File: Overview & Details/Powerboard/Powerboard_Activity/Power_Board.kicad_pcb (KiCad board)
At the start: 4 copper layers, 198 x 120.6 mm, 51 parts, among them J1 Jack-DC, J2 Screw_Terminal_01x04, J3 Screw_Terminal_01x04, J4 Screw_Terminal_01x02, J5 Screw_Terminal_01x02, U1 LM2576S-ADJ, U2 LM2576S-ADJ, U3 LM2576S-ADJ, U4 LM2576S-ADJ, U5 MAX735CSA

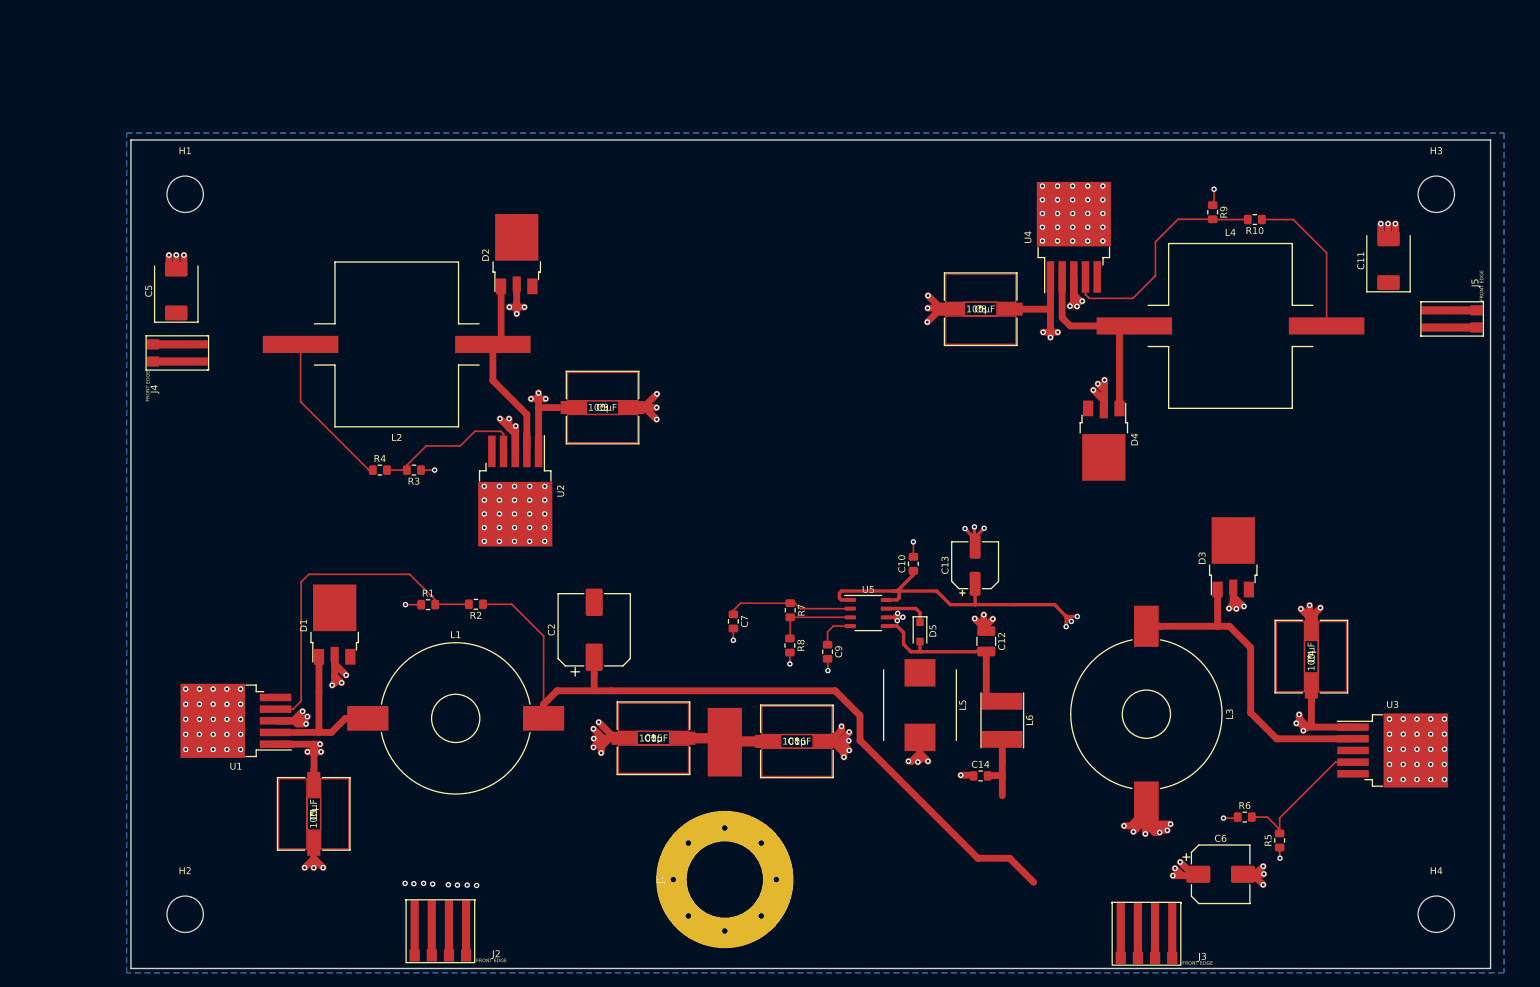
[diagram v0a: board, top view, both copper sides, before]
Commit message: Finish powerboard design
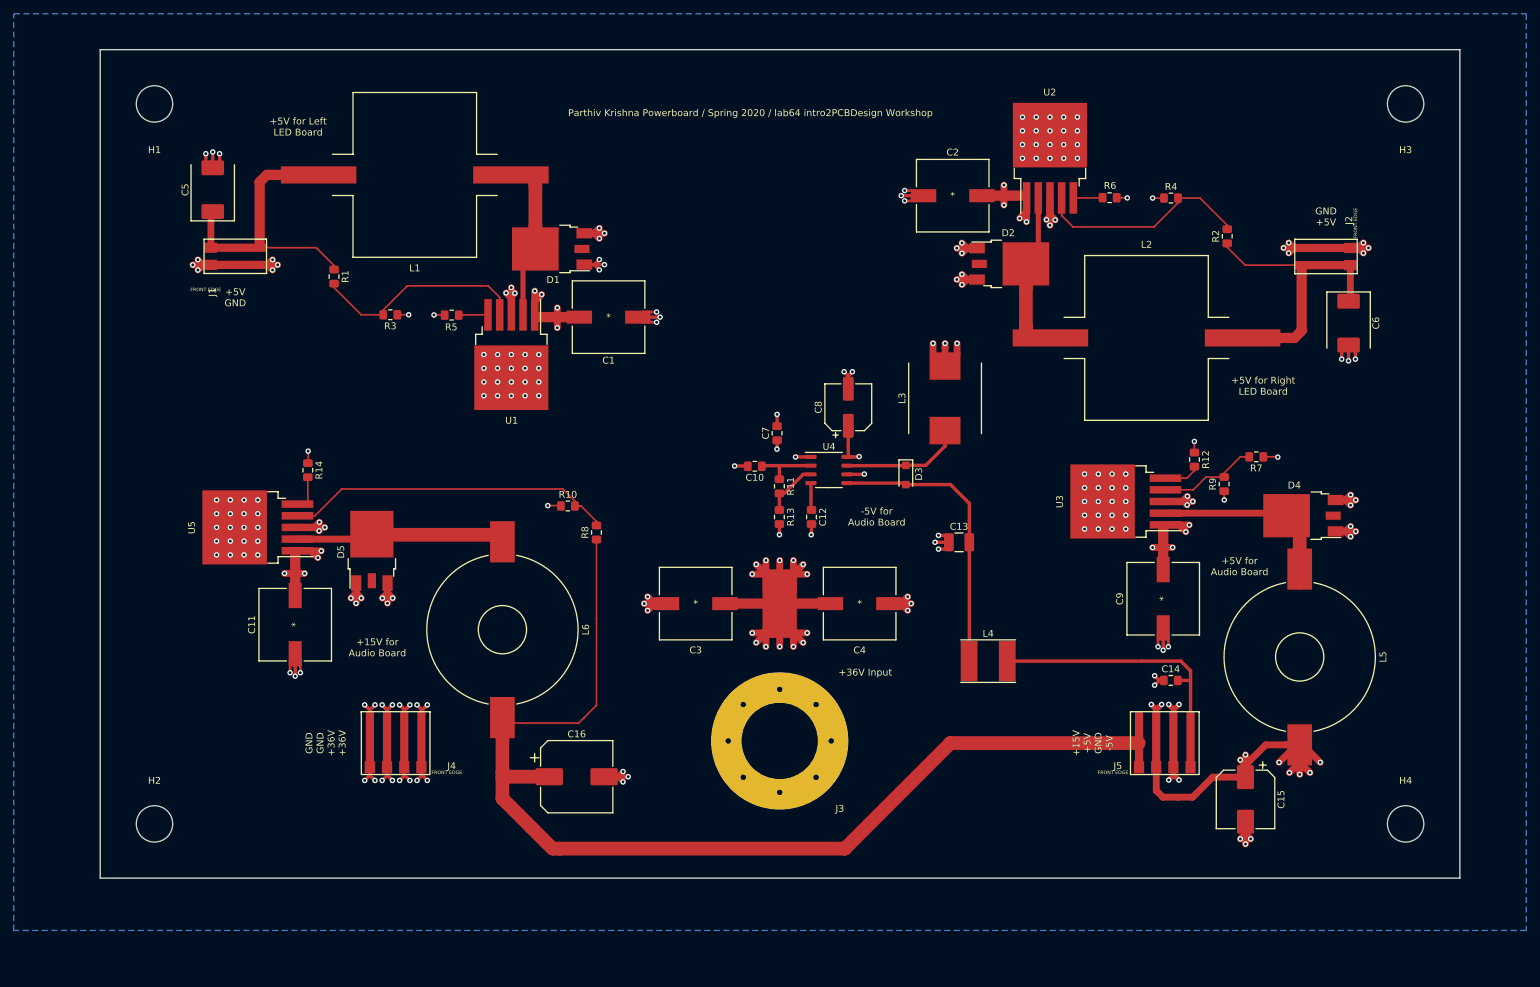
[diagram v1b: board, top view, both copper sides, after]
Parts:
- added R11: 130kΩ, Resistor_SMD:R_0805_2012Metric_Pad1.15x1.40mm_HandSolder, F.Cu at (149.0, 97.4)
- added R12: 20kΩ, Resistor_SMD:R_0805_2012Metric_Pad1.15x1.40mm_HandSolder, F.Cu at (209.5, 93.5)
- added R13: 300kΩ, Resistor_SMD:R_0805_2012Metric_Pad1.15x1.40mm_HandSolder, F.Cu at (149.0, 101.9)
- added R14: 20kΩ, Resistor_SMD:R_0805_2012Metric_Pad1.15x1.40mm_HandSolder, F.Cu at (80.4, 95.1)
- C10: value 1μF@10V -> 10μF@16V
- C11: value 1000µF -> 100µF; footprint Capacitor_Tantalum_SMD:CP_EIA-7361-438_AVX-U_Pad2.18x3.30mm_HandSolder -> Powerboard:PCR1J101MCL1GS
- C12: value 100μF@10V -> 82pF; footprint Capacitor_SMD:C_1210_3225Metric_Pad1.42x2.65mm_HandSolder -> Capacitor_SMD:C_0805_2012Metric_Pad1.15x1.40mm_HandSolder
- C13: value 47μF@10V -> 100μF@10V; footprint Capacitor_SMD:CP_Elec_6.3x5.7 -> Capacitor_SMD:C_1210_3225Metric_Pad1.42x2.65mm_HandSolder
- C15: value 100μF -> 330µF; footprint Powerboard:PCR1J101MCL1GS -> Capacitor_SMD:CP_Elec_8x10
- C16: value 100μF -> 68µF; footprint Powerboard:PCR1J101MCL1GS -> Capacitor_SMD:CP_Elec_10x10
- C2: value 68µF -> 100µF; footprint Capacitor_SMD:CP_Elec_10x10 -> Powerboard:PCR1J101MCL1GS
- C3, C4: value 100µF -> 100μF
- C6: value 330µF -> 1000µF; footprint Capacitor_SMD:CP_Elec_8x10 -> Capacitor_Tantalum_SMD:CP_EIA-7361-438_AVX-U_Pad2.18x3.30mm_HandSolder
- C7: value 10μF@16V -> 1μF@10V
- C8: value 100µF -> 47μF@10V; footprint Powerboard:PCR1J101MCL1GS -> Capacitor_SMD:CP_Elec_6.3x5.7
- C9: value 82pF -> 100µF; footprint Capacitor_SMD:C_0805_2012Metric_Pad1.15x1.40mm_HandSolder -> Powerboard:PCR1J101MCL1GS
- D3: value VS-MURD620CT-M3 -> PMEG2010AEH; footprint Powerboard:TO-252AA_TabPin4 -> Diode_SMD:D_SOD-123F
- D5: value PMEG2010AEH -> VS-MURD620CT-M3; footprint Diode_SMD:D_SOD-123F -> Powerboard:TO-252AA_TabPin4
- J1: value Jack-DC -> Screw_Terminal_01x02; footprint Powerboard:BarrelJack_Power_2.1x5.5mm_11mmThruHole_PanelMount -> Powerboard:AVX-Wire-To-Board-1x2
- J2: value Screw_Terminal_01x04 -> Screw_Terminal_01x02; footprint Powerboard:AVX-Wire-To-Board-1x4 -> Powerboard:AVX-Wire-To-Board-1x2
- J3: value Screw_Terminal_01x04 -> Jack-DC; footprint Powerboard:AVX-Wire-To-Board-1x4 -> Powerboard:BarrelJack_Power_2.1x5.5mm_11mmThruHole_PanelMount
- J4, J5: value Screw_Terminal_01x02 -> Screw_Terminal_01x04; footprint Powerboard:AVX-Wire-To-Board-1x2 -> Powerboard:AVX-Wire-To-Board-1x4
- L1: value 470µH -> 100µH; footprint Powerboard:L_Toroid_Horizontal_D21.8mm_P19.60mm_Bourns_2100 -> Powerboard:Eaton_CTX100-2-52-R
- L3: value 330µH -> 10μH; footprint Powerboard:L_Toroid_Horizontal_D21.8mm_P19.60mm_Bourns_2100 -> Powerboard:L_Taiyo-Yuden_NR-10050_9.8x10.0mm_HandSoldering
- L4: value 100µH -> 22μH; footprint Powerboard:Eaton_CTX100-2-52-R -> Powerboard:L_Taiyo-Yuden_NR-60xx_HandSoldering
- L5: value 10μH -> 330µH; footprint Powerboard:L_Taiyo-Yuden_NR-10050_9.8x10.0mm_HandSoldering -> Powerboard:L_Toroid_Horizontal_D21.8mm_P19.60mm_Bourns_2100
- L6: value 22μH -> 470µH; footprint Powerboard:L_Taiyo-Yuden_NR-60xx_HandSoldering -> Powerboard:L_Toroid_Horizontal_D21.8mm_P19.60mm_Bourns_2100
- R1: value 1.02kΩ -> 3.09kΩ
- R10: value 3.09kΩ -> 1.02kΩ
- R2: value 11.50kΩ -> 3.09kΩ
- R4: value 3.09kΩ -> 1.0kΩ
- R5: value 1.0kΩ -> 20kΩ
- R6: value 3.09kΩ -> 20kΩ
- R7: value 130kΩ -> 3.09kΩ
- R8: value 300kΩ -> 11.50kΩ
- U4: value LM2576S-ADJ -> MAX735CSA; footprint Package_TO_SOT_SMD:TO-263-5_TabPin3 -> Package_SO:SOP-8_3.9x4.9mm_P1.27mm
- U5: value MAX735CSA -> LM2576S-ADJ; footprint Package_SO:SOP-8_3.9x4.9mm_P1.27mm -> Package_TO_SOT_SMD:TO-263-5_TabPin3
- moved J2 169.3 mm to (232.2, 65.2), turned to 90 degrees
- moved C11 167.8 mm to (78.5, 117.6), turned to 270 degrees
- moved R5 142.8 mm to (101.3, 72.5), turned to 0 degrees
- moved R2 121.8 mm to (214.3, 61.0), turned to 90 degrees
- moved R4 121.8 mm to (206.1, 55.4)
- moved J1 118.6 mm to (66.3, 62.7), turned to 270 degrees
- moved L2 109.2 mm to (202.5, 75.8), turned to 0 degrees
- moved R10 108.4 mm to (118.2, 100.3), turned to 0 degrees
- moved R6 92.3 mm to (197.1, 55.4), turned to 180 degrees
- moved U2 91.7 mm to (188.4, 49.7), turned to 90 degrees
- moved U5 89.8 mm to (73.1, 103.4), turned to 180 degrees
- moved C15 86.7 mm to (216.9, 143.0), turned to 270 degrees
- moved C1 84.1 mm to (124.2, 72.8), turned to 0 degrees
- moved C6 82.4 mm to (231.9, 73.7), turned to 270 degrees
- moved C2 82.0 mm to (174.3, 55.1), turned to 180 degrees
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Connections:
- C10 pad 1: +5VA -> Net-(C10-Pad1)
- C11 pad 1: +5VR -> +36V
- C12 pad 1: GNDS -> Net-(C12-Pad1)
- C12 pad 2: Net-(C12-Pad2) -> GNDS
- C13 pad 1: +5VA -> GNDS
- C13 pad 2: GNDS -> Net-(C13-Pad2)
- C15 pad 1: +36V -> +5VA
- C16 pad 1: +36V -> +15V
- C2 pad 1: +15V -> +36V
- C6 pad 1: +5VA -> +5VR
- C7 pad 1: Net-(C7-Pad1) -> +5VA
- C8 pad 1: +36V -> +5VA
- C9 pad 1: Net-(C9-Pad1) -> +36V
- D3 pad 2: GNDS -> Net-(C13-Pad2)
- D5 pad 2: Net-(C12-Pad2) -> GNDS
- J1 pad 1: GNDS -> +5VL
- J1 pad 2: +36V -> GNDS
- J2 pad : (no net) -> +5VR
- J2 pad 1: GNDS -> +5VR
- J3 pad 1: +15V -> GNDS
- J3 pad 2: +5VA -> +36V
- J4 pad : (no net) -> GNDS
- J4 pad 1: +5VL -> GNDS
- J5 pad : (no net) -> -5VA
- J5 pad 1: +5VR -> +15V
- J5 pad 2: GNDS -> +5VA
- J5 pad 3: (no net) -> GNDS
- J5 pad 4: (no net) -> -5VA
- L1 pad 2: +15V -> +5VL
- L2 pad 2: +5VL -> +5VR
- L3 pad 2: +5VA -> GNDS
- L4 pad 1: Net-(D4-Pad1) -> Net-(C13-Pad2)
- L4 pad 2: +5VR -> -5VA
- L5 pad 1: Net-(D5-Pad1) -> Net-(D4-Pad1)
- L5 pad 2: GNDS -> +5VA
- L6 pad 1: Net-(C12-Pad2) -> Net-(D5-Pad1)
- L6 pad 2: -5VA -> +15V
- R1 pad 1: GNDS -> +5VL
- R10 pad 1: +5VR -> GNDS
- R2 pad 1: +15V -> +5VR
- R2 pad 2: Net-(R1-Pad2) -> Net-(R2-Pad2)
- R3 pad 2: Net-(R3-Pad2) -> Net-(R1-Pad2)
- R4 pad 1: +5VL -> GNDS
- R4 pad 2: Net-(R3-Pad2) -> Net-(R2-Pad2)
- R6 pad 1: +5VA -> GNDS
- R6 pad 2: Net-(R5-Pad2) -> Net-(R6-Pad2)
- R7 pad 1: Net-(C7-Pad1) -> +5VA
- R8 pad 1: Net-(R7-Pad2) -> +15V
- R8 pad 2: GNDS -> Net-(R10-Pad2)
- R9 pad 2: Net-(R10-Pad2) -> Net-(R7-Pad2)
- U1 pad 5: Net-(U1-Pad5) -> Net-(R5-Pad2)
- U2 pad 4: Net-(R3-Pad2) -> Net-(R2-Pad2)
- U2 pad 5: Net-(U2-Pad5) -> Net-(R6-Pad2)
- U3 pad 2: Net-(D3-Pad1) -> Net-(D4-Pad1)
- U3 pad 4: Net-(R5-Pad2) -> Net-(R7-Pad2)
- U4 pad 1: +36V -> +5VA
- U4 pad 2: Net-(D4-Pad1) -> Net-(C10-Pad1)
- U4 pad 3: GNDS -> Net-(R11-Pad2)
- U4 pad 4: Net-(R10-Pad2) -> Net-(C12-Pad1)
- U4 pad 5: Net-(U4-Pad5) -> Net-(C13-Pad2)
- U5 pad 1: +5VA -> +36V
- U5 pad 2: Net-(C7-Pad1) -> Net-(D5-Pad1)
- U5 pad 3: Net-(R7-Pad2) -> GNDS
- U5 pad 4: Net-(C9-Pad1) -> Net-(R10-Pad2)
- U5 pad 5: Net-(C12-Pad2) -> Net-(R14-Pad2)
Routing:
- net +36V: track 78.1 -> 193.2 mm, vias 16 -> 38
- net GNDS: track 235.5 -> 306.2 mm, vias 177 -> 193
- net +15V: track 115.5 -> 168.5 mm
- net Net-(C13-Pad2): track 0.00 -> 42.5 mm
- net -5VA: track 10.4 -> 43.2 mm
- net Net-(R2-Pad2): track 0.00 -> 31.7 mm
- net Net-(D3-Pad1): track 47.8 -> 17.8 mm
- net Net-(C12-Pad2): track 28.6 -> 0.00 mm
- net Net-(D5-Pad1): track 6.55 -> 33.1 mm
- net +5VR: track 22.1 -> 48.3 mm
- net +5VL: track 23.0 -> 47.9 mm
- net Net-(R3-Pad2): track 22.4 -> 0.00 mm
- net +5VA: track 96.1 -> 77.1 mm
- net Net-(C7-Pad1): track 18.4 -> 0.00 mm
- net Net-(R1-Pad2): track 48.7 -> 31.7 mm
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- added copper zone on In2.Cu, net +5VA
- removed copper zone on In2.Cu, net (none)
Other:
- board size 198 x 120.6 mm -> 198 x 120.7 mm
- board text added: "+15V +5V GND -5V"
- board text added: "+15V for Audio Board"
- board text added: "+36V Input"
- board text added: "+36V ⎓ 1.83A Parthiv Krishna UberRadio"
- board text added: "+5V GND"
- board text added: "+5V for Audio Board"
- board text added: "+5V for Left LED Board"
- board text added: "+5V for Right LED Board"
- board text added: "-5V for Audio Board"
- board text added: "2"
- board text added: "3"
- board text added: "GND +5V"
- board text added: "GND GND +36V +36V"
- board text added: "Parthiv Krishna Powerboard / Spring 2020 / lab64 intro2PCBDesign Workshop"
